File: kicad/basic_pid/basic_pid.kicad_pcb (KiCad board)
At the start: 4 copper layers, 152.4 x 101.6 mm, 121 parts, among them J1 Input A, J2 Input B / Setpoint, J3 Monitor, J4 Output, J5 Screw_Terminal_01x04, J6 Screw_Terminal_01x03, SW1 SW_DPDT_x2, SW10 SW_DPDT_x2, SW2 SW_DPDT_x2, SW3 SW_DPDT_x2, SW4 SW_SP4T, SW5 SW_DPDT_x2, SW6 SW_SP4T, SW7 SW_SP4T, SW8 SW_SP4T, SW9 SW_SP4T, U1 LM4040DBZ-5, U10 OPA189, U11 OPA189, U12 OPA189, U13 BUF634A, U14 LM2940CS-12/NOPB, U15 LM2990SX-12, U16 LM317_TO-252, U2 LM4040DBZ-5, U3 LT1167, U4 LT1167, U5 OPA189, U6 OPA189, U7 OPA189, U8 BUF634A, U9 OPA189

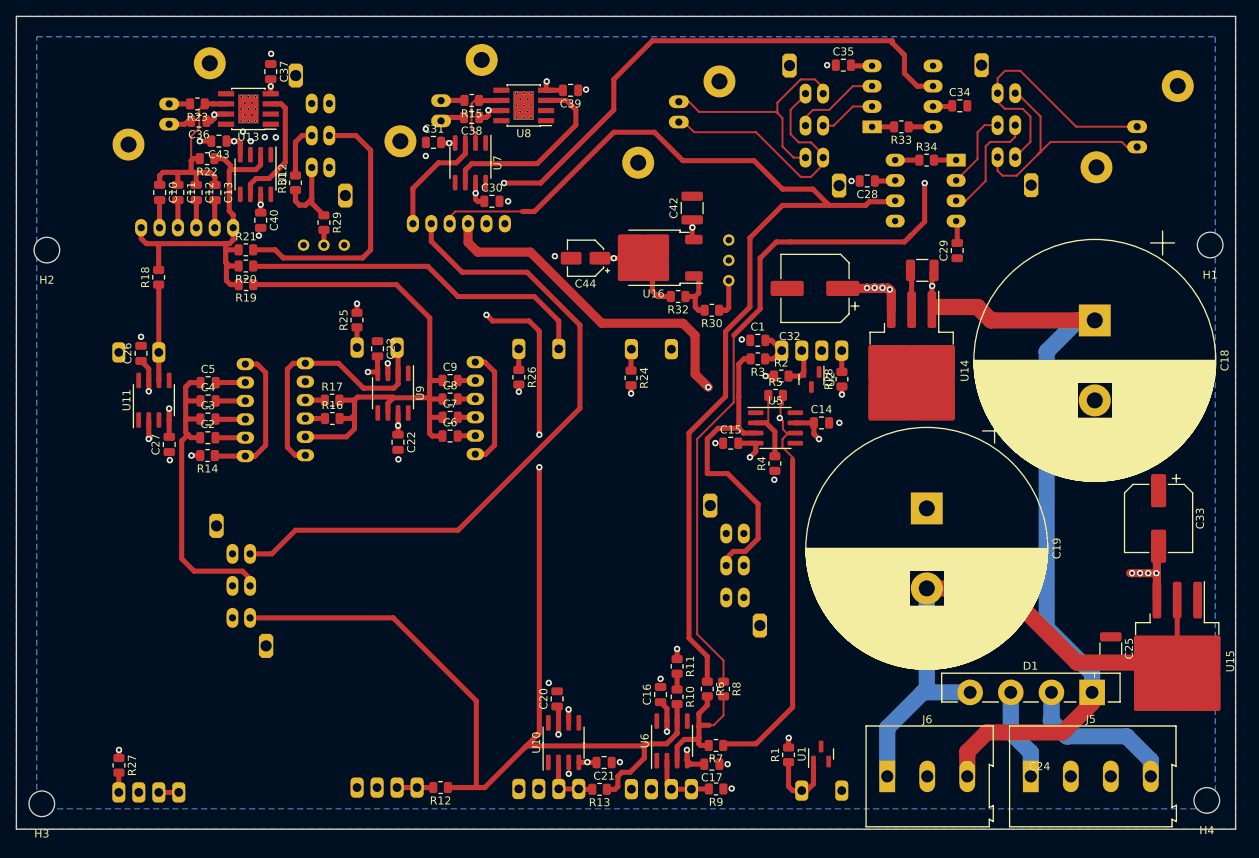
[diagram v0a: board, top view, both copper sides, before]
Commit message: version sent to Advanced Circuits and OSHStencils
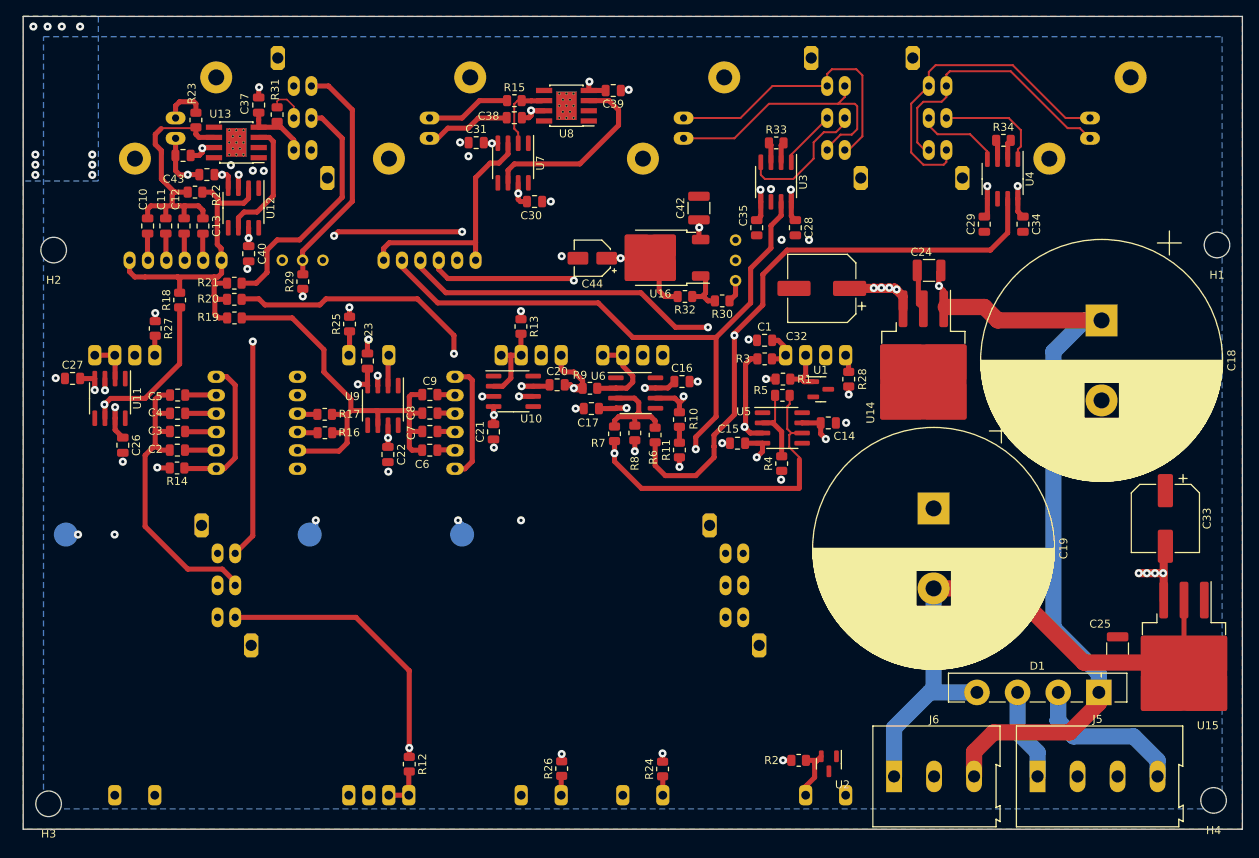
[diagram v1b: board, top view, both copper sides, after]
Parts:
- added LOGO3: JQI-LOGOSILK, lib:JQI_LOGO_NEGATIVE-SILKSCREEN, B.Cu at (250.6, 80.5)
- added TP1: TestPoint, TestPoint:TestPoint_Pad_D3.0mm, B.Cu at (137.4, 90.2)
- added TP2: TestPoint, TestPoint:TestPoint_Pad_D3.0mm, B.Cu at (156.5, 90.2)
- added TP3: TestPoint, TestPoint:TestPoint_Pad_D3.0mm, B.Cu at (106.9, 90.2)
- U3, U4: value LT1167 -> INA849; footprint Package_DIP:DIP-8_W7.62mm_LongPads -> Package_SO:SOIC-8_3.9x4.9mm_P1.27mm; moved to F.Cu
- moved R13 58.7 mm to (163.8, 64.2), turned to -90 degrees
- moved R27 54.8 mm to (118.1, 64.4)
- moved R9 52.5 mm to (172.4, 71.9), turned to 0 degrees
- moved R26 49.2 mm to (168.9, 119.4), turned to 90 degrees
- moved R24 49.0 mm to (181.5, 119.5), turned to 90 degrees
- moved R2 48.1 mm to (198.5, 118.4)
- moved U2 48.1 mm to (202.3, 118.8)
- moved R1 47.0 mm to (196.6, 70.7), turned to 180 degrees
- moved C17 46.9 mm to (172.6, 74.4), turned to 0 degrees
- moved U1 45.6 mm to (201.3, 72.0), turned to 0 degrees
- moved U10 44.4 mm to (162.9, 72.3), turned to 0 degrees
- moved U6 43.7 mm to (178.2, 72.5), turned to 0 degrees
- moved C21 43.6 mm to (160.4, 77.3), turned to 90 degrees
- moved R7 41.0 mm to (175.5, 77.6), turned to 90 degrees
- moved C20 39.3 mm to (168.3, 71.5), turned to 0 degrees
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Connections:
- net Net-(D1--) renamed V-_unreg
- net Net-(J5-Pin_1) renamed /Supply_and_filtering/black
- net Net-(J5-Pin_4) renamed /Supply_and_filtering/yellow
- RV1 pad 1: Net-(U2-A) -> Net-(U1-K)
- RV1 pad 3: Net-(U1-K) -> Net-(U2-A)
- U3 pad 1: Net-(R33-Pad2) -> Net-(SW1A-B)
- U3 pad 2: Net-(SW1B-B) -> Net-(R33-Pad2)
- U3 pad 3: Net-(SW1A-B) -> Net-(R33-Pad1)
- U3 pad 4: -12V -> Net-(SW1B-B)
- U3 pad 5: GND -> -12V
- U3 pad 6: Input_A -> GND
- U3 pad 7: +12V -> Input_A
- U3 pad 8: Net-(R33-Pad1) -> +12V
- U4 pad 1: Net-(R34-Pad2) -> Net-(SW2A-B)
- U4 pad 2: Net-(SW2B-B) -> Net-(R34-Pad2)
- U4 pad 3: Net-(SW2A-B) -> Net-(R34-Pad1)
- U4 pad 4: -12V -> Net-(SW2B-B)
- U4 pad 5: GND -> -12V
- U4 pad 6: Input_B -> GND
- U4 pad 7: +12V -> Input_B
- U4 pad 8: Net-(R34-Pad1) -> +12V
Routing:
- net Input_A: track 264.0 -> 139.4 mm, vias 2 -> 3
- net Net-(R18-Pad1): track 12.0 -> 75.8 mm, vias 0 -> 3
- net Net-(U11--): track 57.4 -> 23.3 mm, vias 2 -> 1
- net GND: track 13.6 -> 40.0 mm, vias 27 -> 40
- net Internal_setpoint: track 106.2 -> 84.0 mm
- net Input_B: track 136.3 -> 117.8 mm, vias 0 -> 2
- net Error_signal: track 158.7 -> 142.9 mm
- net Net-(R20-Pad1): track 91.6 -> 103.3 mm, vias 1 -> 4
- net Net-(SW1B-B): track 7.11 -> 17.0 mm
- net Net-(R11-Pad1): track 39.0 -> 47.6 mm
- net Net-(J3-In): track 2.93 -> 10.6 mm
- net Net-(U13-OUT): track 25.9 -> 33.2 mm
- net Net-(J2-In): track 34.4 -> 40.9 mm
- net Net-(U6-+): track 18.7 -> 13.1 mm
- net Net-(SW10A-C): track 24.9 -> 29.5 mm
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- added copper zone on B.Cu, net GND
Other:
- board text added: "A"
- board text added: "B"
- board text added: "Bandwidth-limit"
- board text added: "Black"
- board text added: "D"
- board text added: "Derivative tau"
- board text added: "Disable offset"
- board text added: "E"
- board text added: "Integral control"
- board text added: "Integral tau"
- board text added: "Orange"
- board text added: "Polarity"
- board text added: "Red"
- board text added: "Rev 1.0"
- board text added: "SP"
- board text added: "Skip-setpoint"
- board text added: "Teach me a PID"
- board text added: "V+ unreg"
- board text added: "V- unreg"
- board text added: "Yellow"
